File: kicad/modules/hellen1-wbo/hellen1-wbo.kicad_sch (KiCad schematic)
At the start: 59 parts, among them J1 Conn_01x08, J3 Conn_01x08, J4 FTSH-107-01-F-DV-K, Q1 BTS3028, U1 MCP6004, U2 STM32F042K6Tx, U3 REF3033, U5 AD8628, U9 XC6206P332MR

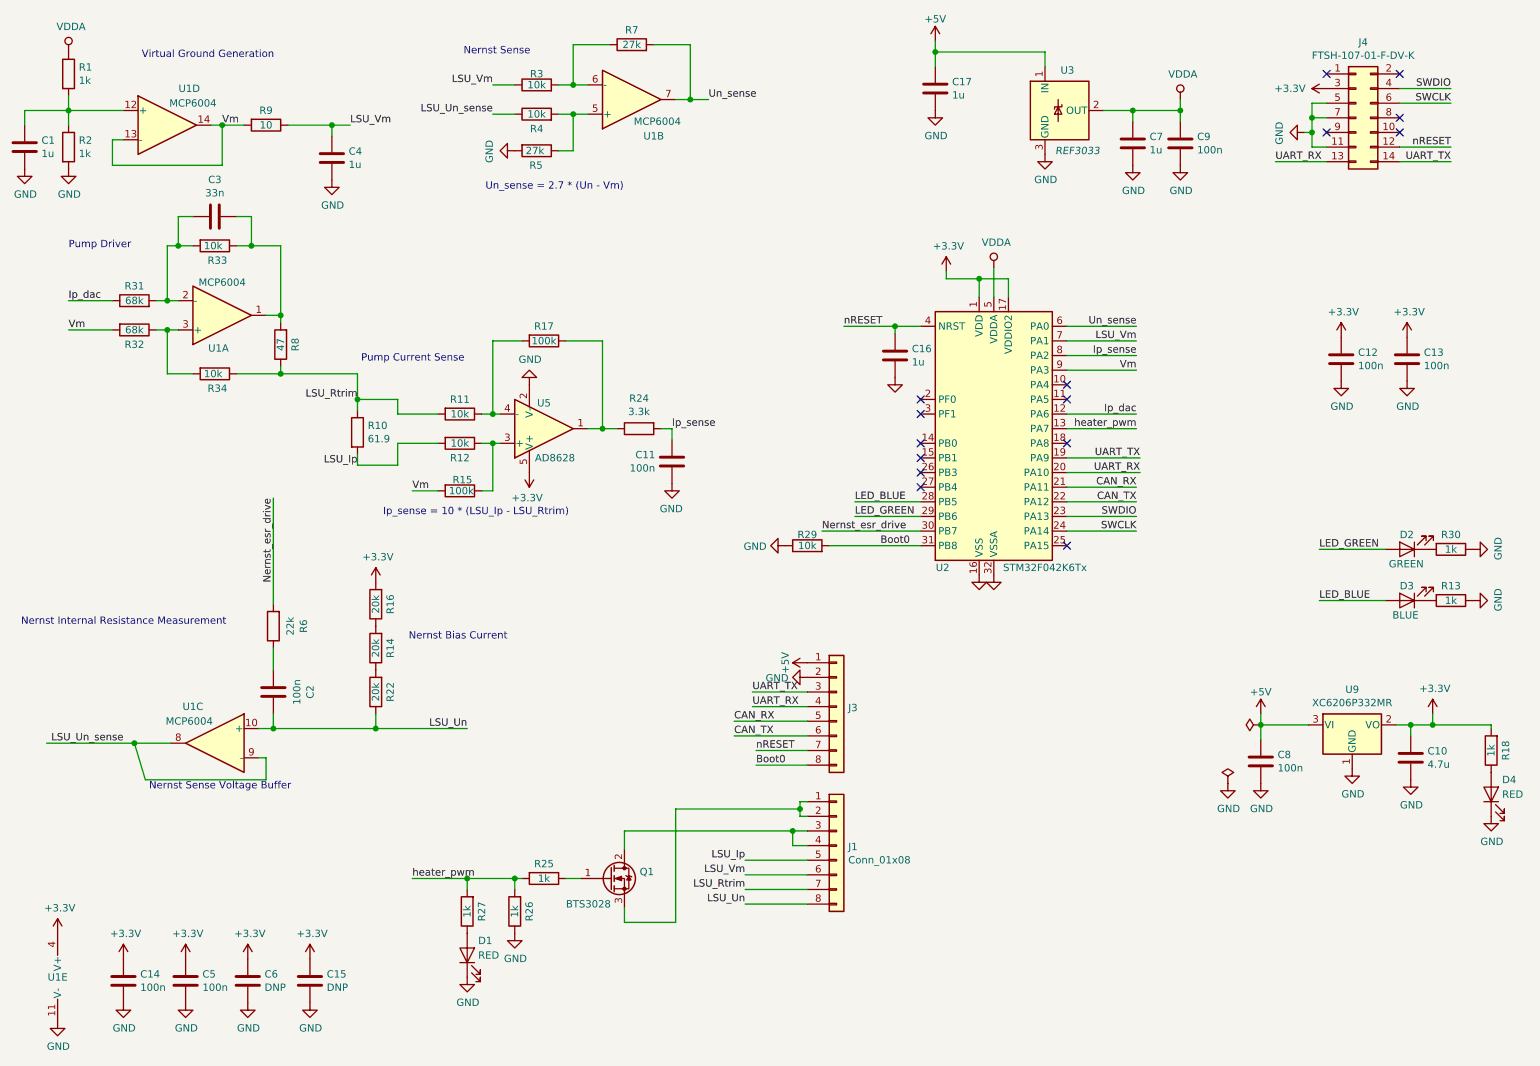
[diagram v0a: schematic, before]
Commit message: update wbo module (kicad source files)
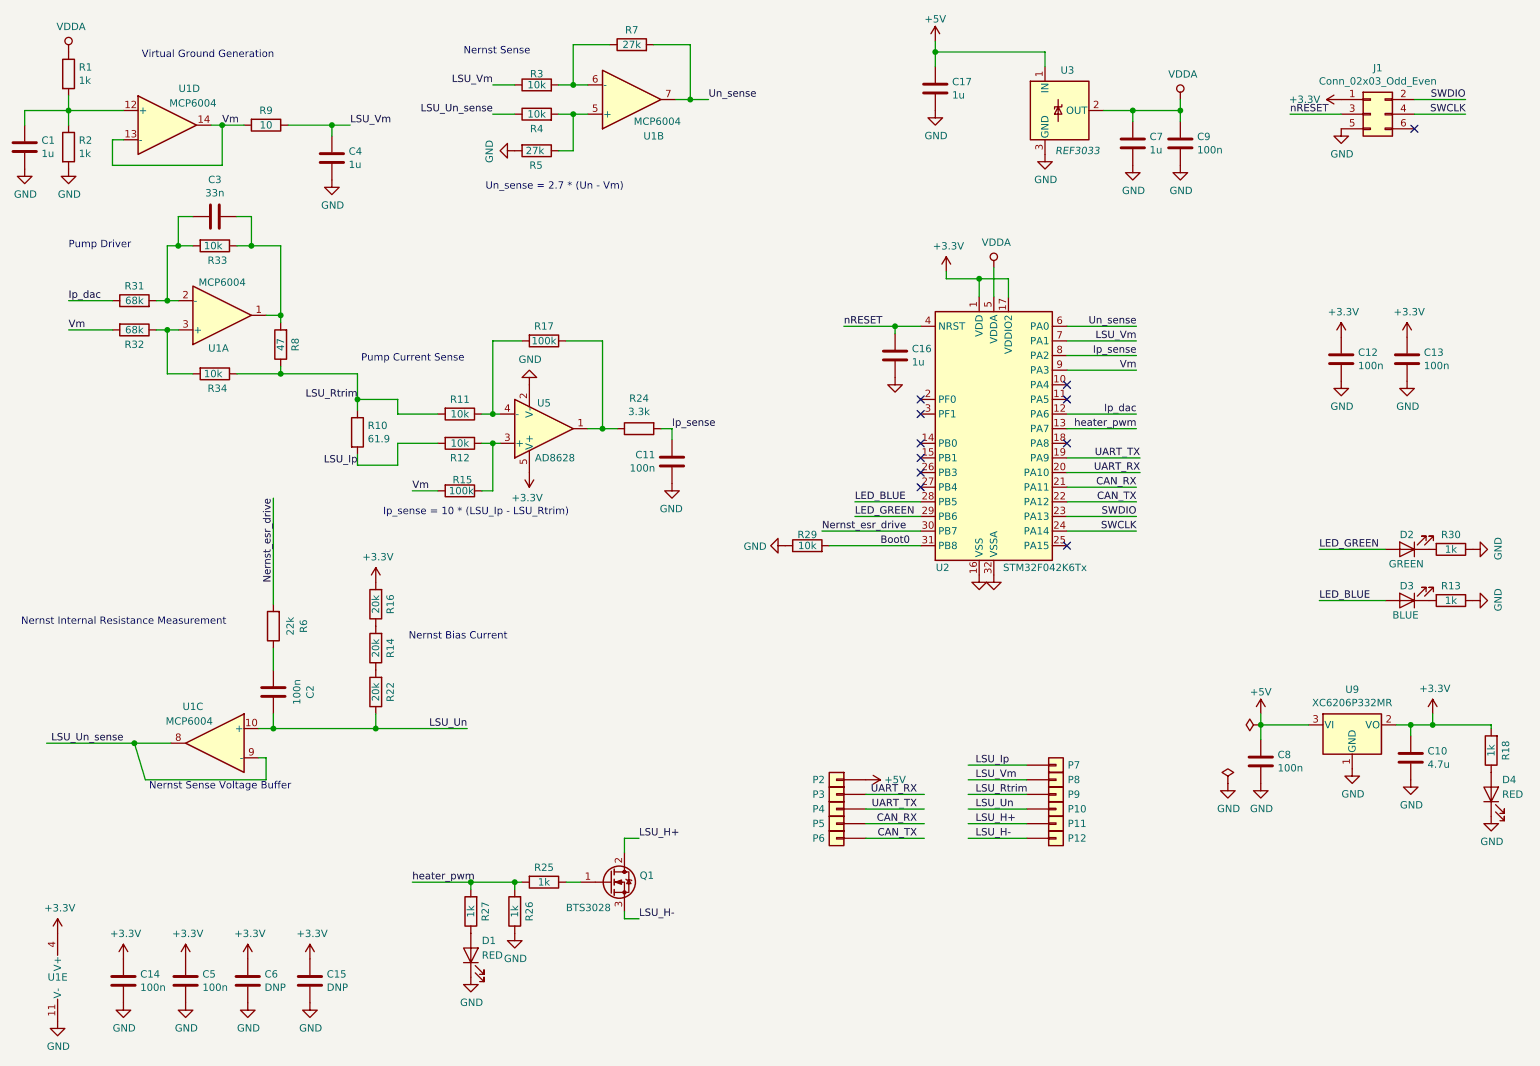
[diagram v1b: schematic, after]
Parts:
- removed J1, J3: Conn_01x08, Connector_PinHeader_2.54mm:PinHeader_1x08_P2.54mm_Vertical, symbol hellen1-wbo-rescue:Conn_01x08-Connector_Generic
- removed J4: FTSH-107-01-F-DV-K, Connector_PinHeader_1.27mm:PinHeader_2x07_P1.27mm_Vertical_SMD, symbol hellen1-wbo-rescue:Conn_02x07_Odd_Even-Connector_Generic
- added J1: Conn_02x03_Odd_Even, Connector:Tag-Connect_TC2030-IDC-NL_2x03_P1.27mm_Vertical, symbol Connector_Generic:Conn_02x03_Odd_Even
- added P10, P2, P3, P4, P5, P6, P7, P8, P9: Pad, footprints:MODULE-PAD-SMD_0.25x0.5, symbol hellen-one-common:Pad
- added P11, P12: Pad, footprints:MODULE-PAD-SMD_3.0, symbol hellen-one-common:Pad
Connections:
- net +3V3: now also J1.1 (Pin_1)
- net +5V: now also P2.1 (Pin_1)
- net CAN_RX: now also P5.1 (Pin_1)
- net CAN_TX: now also P6.1 (Pin_1)
- net GND: now also J1.5 (Pin_5)
- net LSU_Ip: now also P7.1 (Pin_1)
- net LSU_Rtrim: now also P9.1 (Pin_1)
- net LSU_Un: now also P10.1 (Pin_1)
- net LSU_Vm: now also P8.1 (Pin_1)
- net SWCLK: now also J1.4 (Pin_4)
- net SWDIO: now also J1.2 (Pin_2)
- net UART_RX: now also P3.1 (Pin_1)
- net UART_TX: now also P4.1 (Pin_1)
- net nRESET: now also J1.3 (Pin_3)
- net LSU_H+: now reaches Q1.2 (D)
- net LSU_H+: now also P11.1 (Pin_1)
- net LSU_H-: now reaches Q1.3 (S)
- net LSU_H-: now also P12.1 (Pin_1)
- no-connect marks 15 -> 11
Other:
- moved on the sheet: D1, Q1, R25, R27
